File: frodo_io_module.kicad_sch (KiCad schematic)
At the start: 150 parts, among them J1 Conn_02x04_Top_Bottom, J10 JST-GH 4Pin, J11 JST-GH 4Pin, J14 Conn_02x03_Odd_Even, J16 USB_C_Receptacle_USB2.0, J17 TC2050, J2 Conn_02x10_Odd_Even, J3 Conn_02x04_Top_Bottom, J4 Conn_02x03_Odd_Even, J5 Conn_02x04_Odd_Even, J6 JST-GH 4Pin, J7 JST-GH 4Pin, J8 JST-GH 4Pin, J9 JST-GH 4Pin, SW1 KMR721NGLFS, SW2 KMR721NGLFS, SW3 KMR721NGLFS, U1 L7805, U10 MCP2562-E-SN, U11 TPD4E1U06, U12 INA181A1, U2 L7805, U3 STM32F105RCTx, U4 AZ1117H-ADJ, U5 AZ1117H-ADJ, U6 W25Q128JVP, U7 MCP2562-E-SN, U8 TPD4E1U06, U9 INA181A1, Y1 8MHz 12pF

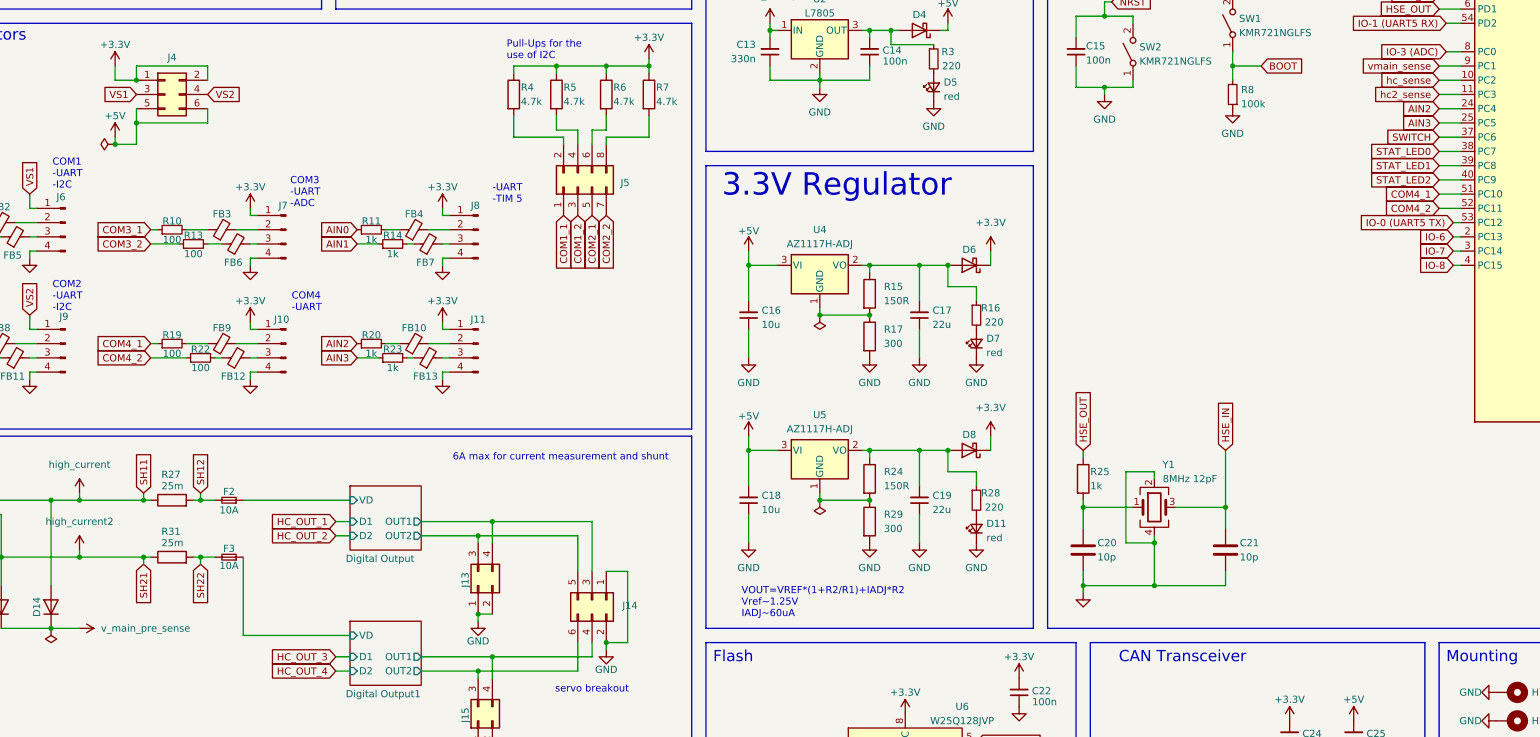
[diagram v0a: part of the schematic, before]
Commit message: more routing
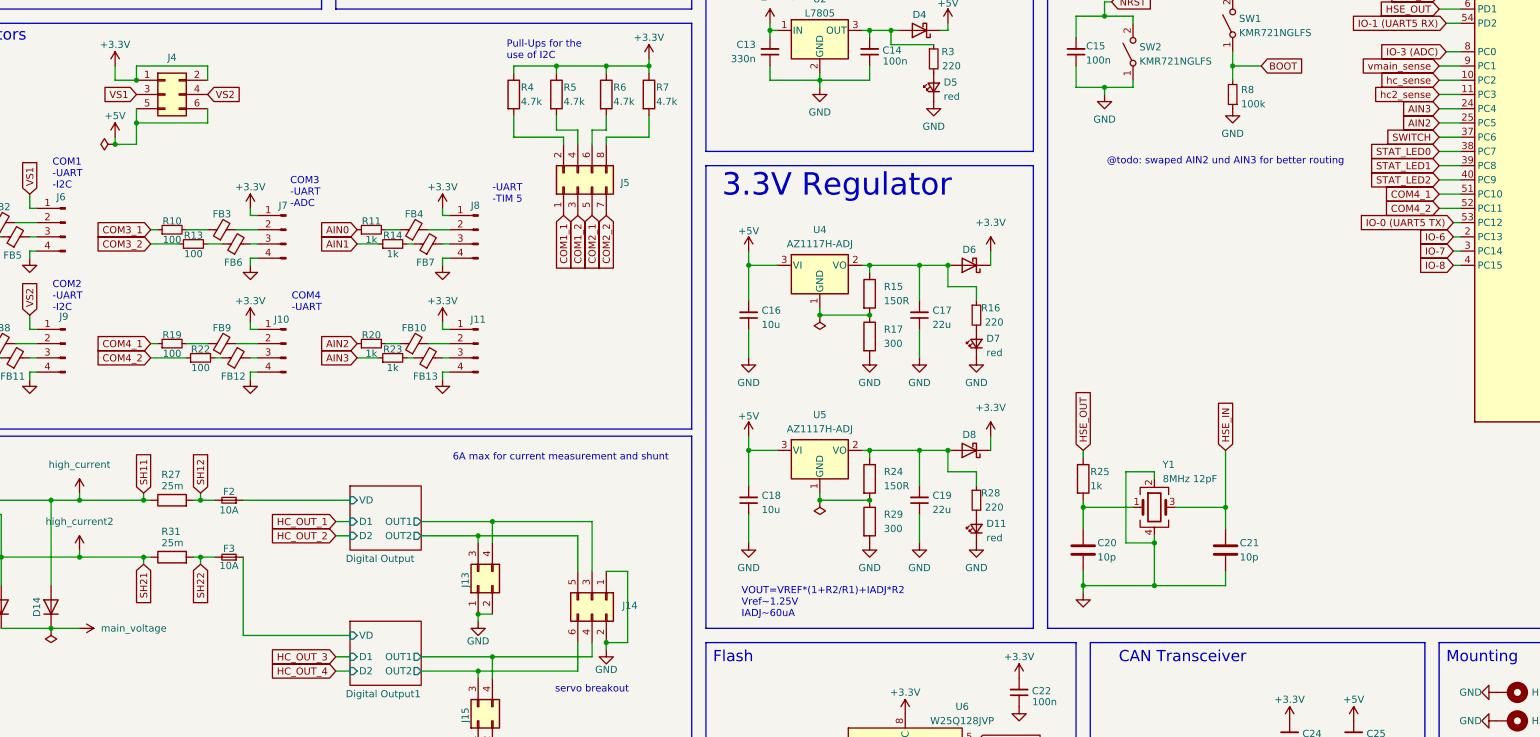
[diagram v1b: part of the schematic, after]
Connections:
- net v_main_pre_sense is gone; now on net main_voltage: D13.1 (K), D14.1 (K)
- net AIN2: now also U3.25 (PC5); no longer U3.24 (PC4)
- net AIN3: now also U3.24 (PC4); no longer U3.25 (PC5)
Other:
- note added: "@todo: swaped AIN2 und AIN3 for better routing"
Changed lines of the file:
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@@
 		)
 	)
+	(text "@todo: swaped AIN2 und AIN3 for better routing"
+		(exclude_from_sim no)
+		(at 261.62 89.408 0)
+		(effects
+			(font
+				(size 1.27 1.27)
+			)
+		)
+	)
 	(text "Isense"
 		(exclude_from_sim no)
@@
 	(global_label "AIN3"
 		(shape input)
-		(at 299.72 82.55 180)
+		(at 299.72 80.01 180)
 		(fields_autoplaced yes)
 		(effects
@@
 		)
 		(property "Intersheetrefs" "${INTERSHEET_REFS}"
-			(at 292.5014 82.55 0)
+			(at 292.5014 80.01 0)
 			(effects
 				(font
@@
 	(global_label "AIN2"
 		(shape input)
-		(at 299.72 80.01 180)
+		(at 299.72 82.55 180)
 		(fields_autoplaced yes)
 		(effects
@@
 		)
 		(property "Intersheetrefs" "${INTERSHEET_REFS}"
-			(at 292.5014 80.01 0)
+			(at 292.5014 82.55 0)
 			(effects
 				(font
@@
 			)
 		)
-		(property "Value" "v_main_pre_sense"
+		(property "Value" "main_voltage"
 			(at 60.96 172.7199 90)
 			(effects
